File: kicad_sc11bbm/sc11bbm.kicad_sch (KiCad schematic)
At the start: 8 parts

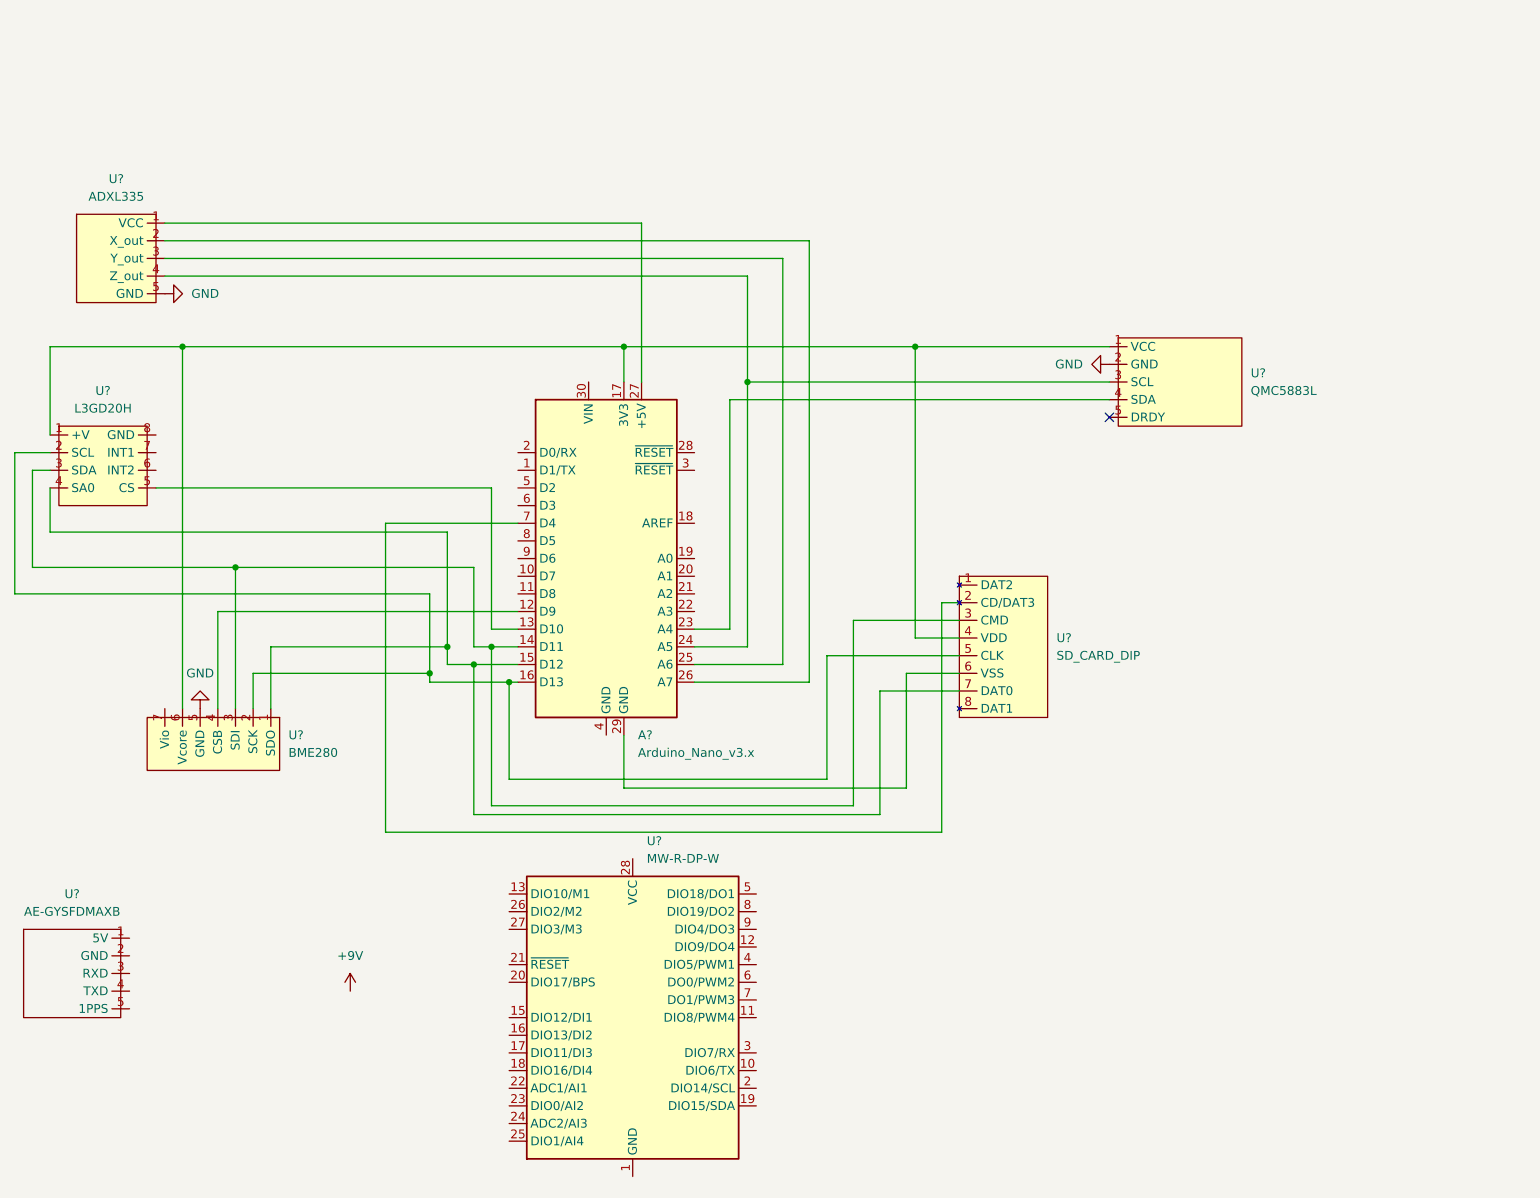
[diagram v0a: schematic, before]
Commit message: Reference settings are not yet
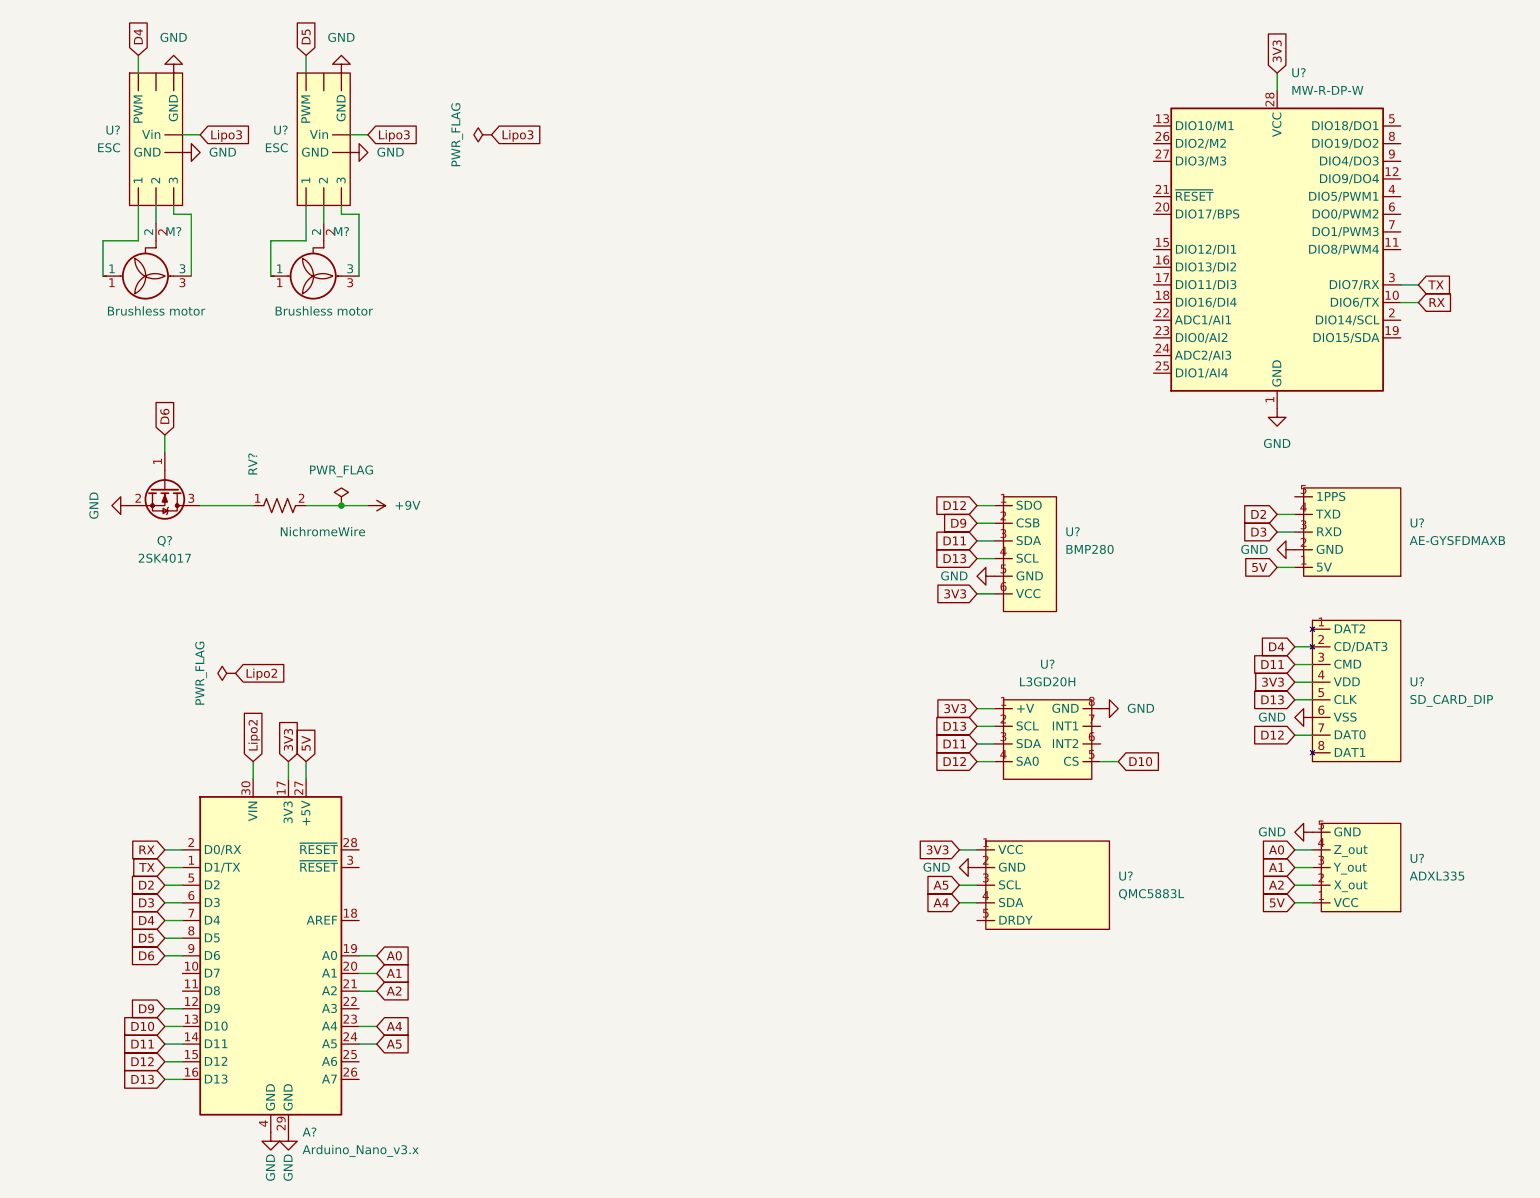
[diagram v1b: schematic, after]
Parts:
- removed U?: BME280, symbol BME280:BME280
- added M? (x2): Brushless motor, symbol Motor:Fan_3pin
- added Q?: 2SK4017, symbol Transistor_FET:2N7002E
- added RV?: NichromeWire, symbol Device:R_Potentiometer_US
- added U?: BMP280, symbol sc11bbm:BMP280
- added U? (x2): ESC, symbol sc11bbm:ESC
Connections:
- net +9V: now also RV?.2
- net GND: now also A?.29 (GND), A?.4 (GND), U?.1 (GND), U?.14 (GND), U?.2 (GND), U?.6 (VSS), U?.8 (GND), Q?.2 (S), U?. (Vin), U?. (Vin), U?.5 (GND)
- net D12: now reaches A?.15 (D12), U?.4 (SA0), U?.7 (DAT0)
- net D12: now also U?.1 (SDO)
- net D13: now reaches A?.16 (D13), U?.2 (SCL), U?.5 (CLK)
- net D13: now also U?.4 (SCL)
- net D11: now reaches A?.14 (D11), U?.3 (CMD), U?.3 (SDA)
- net D11: now also U?.3 (SDA)
- net D9: now reaches A?.12 (D9)
- net D9: now also U?.2 (CSB)
- net 3V3: now reaches A?.17 (3V3), U?.1 (+V), U?.1 (VCC), U?.4 (VDD)
- net 3V3: now also U?.28 (VCC), U?.6 (VCC)
- net 5V: now reaches U?.1 (5V)
- net 5V: now also A?.27 (+5V), U?.1 (VCC)
- net D3: now reaches U?.3 (RXD)
- net D3: now also A?.6 (D3)
- net D2: now reaches U?.4 (TXD)
- net D2: now also A?.5 (D2)
- net A5: now reaches A?.24 (A5), U?.3 (SCL)
- net A5: no longer U?.4 (Z_out)
- net A4: now reaches A?.23 (A4), U?.4 (SDA)
- net RX: now reaches U?.10 (DIO6/TX)
- net RX: now also A?.2 (D0/RX)
- net TX: now reaches U?.3 (DIO7/RX)
- net TX: now also A?.1 (D1/TX)
- net D10: now reaches A?.13 (D10), U?.5 (CS)
- net A0: now reaches A?.19 (A0)
- net A0: now also U?.4 (Z_out)
- net A1: now reaches A?.20 (A1)
- net A1: now also U?.3 (Y_out)
- net A2: now reaches A?.21 (A2)
- net A2: now also U?.2 (X_out)
- net at A?.25 (A6): no longer U?.3 (Y_out)
- net at A?.26 (A7): no longer U?.2 (X_out)
- net Lipo2: now reaches A?.30 (VIN)
- net D4: now reaches A?.7 (D4), U?.2 (CD/DAT3)
- net D4: now also U?. (Vin)
- net D5: now reaches A?.8 (D5)
- net D5: now also U?. (Vin)
- net D6: now reaches A?.9 (D6)
- net D6: now also Q?.1 (G)
- new net: Q?.3 (D), RV?.1
- new net: M?.1, U?. (Vin) (x2)
- new net: M?.2, U?. (Vin) (x2)
- new net: M?.3, U?. (Vin) (x2)
- new net Lipo3: U?. (Vin), U?. (Vin)
- no-connect marks 1 -> 0
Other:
- moved on the sheet: A?, U?
